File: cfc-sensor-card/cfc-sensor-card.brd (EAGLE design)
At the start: 99.8 x 94.6 mm, 146 parts, among them J2 J-SAMTEC-TFM-110-X1-XXX-D-RA, J4 TFM-120-01-L-D-RA, Q2 PMV45EN, Q3 DMP2240UDM, Q4 PMV45EN, Q5 MOSFET-PCH-SOT23-6, Q6 MOSFET-PCH-SOT23-6, Q7 MOSFET-PCH-SOT23-6, Q8 PMV45EN, U1 PIRT1280A1-12, U12 MIC842LYC5, U13 MIC842LYC5, U14 MAX4211FETE, U16 MAX7310ATE, U2 LT3042IMSE#TRPBF, U3 LT3042IMSE#TRPBF, U4 LT3042IMSE#TRPBF, U5 LT3042IMSE#TRPBF, U6 LT3042IMSE#TRPBF, U7 TLC3704IPWRPW14-M, U8 LP2985AIM5-3.3_NOPB, X1 16MHz

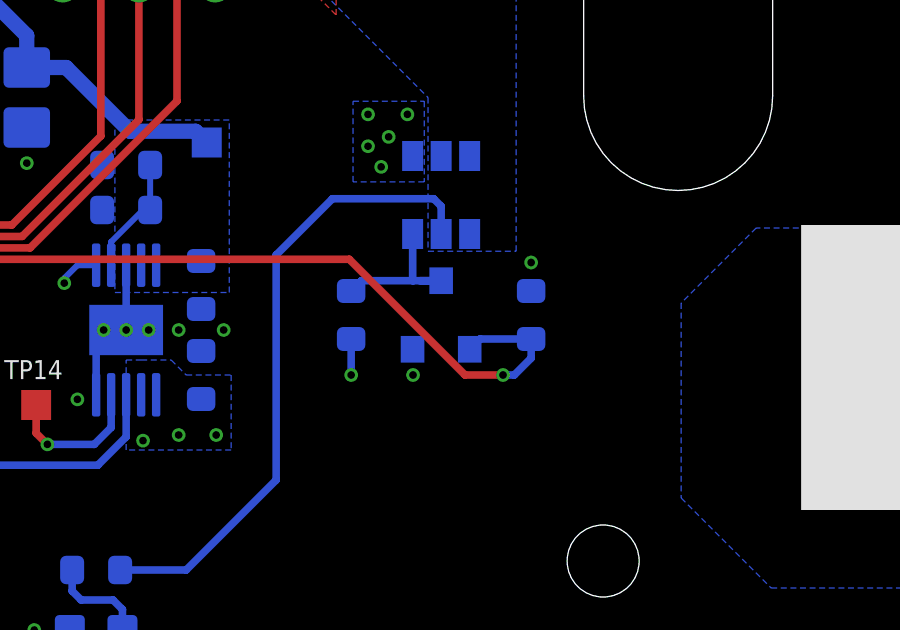
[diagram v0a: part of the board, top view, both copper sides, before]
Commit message: oh god almost done
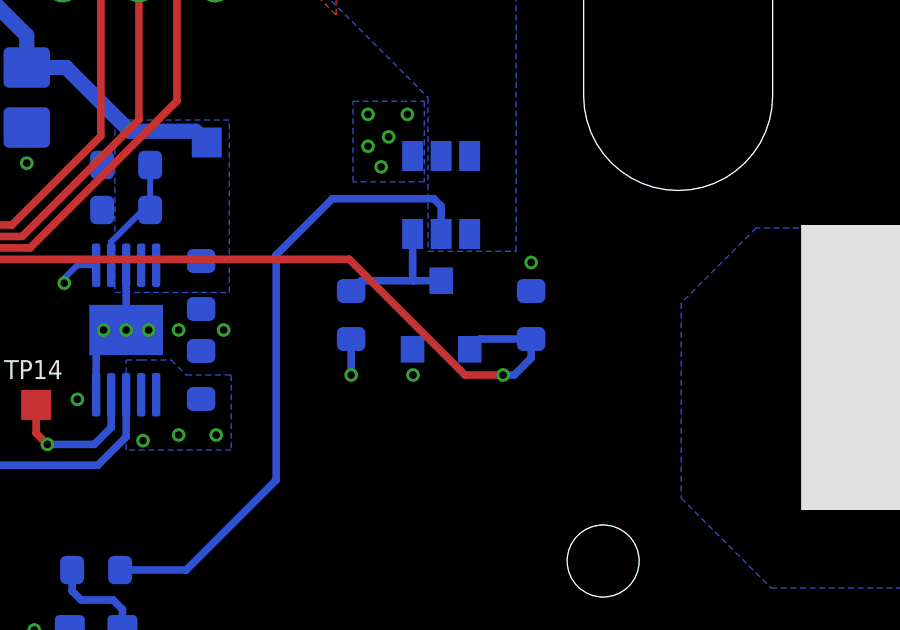
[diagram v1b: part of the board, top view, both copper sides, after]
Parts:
- added U$2: (no value), oresat-misc:ORESAT_ORIENTATION_COPPER
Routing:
- net N$3: track 5.41 -> 4.70 mm
